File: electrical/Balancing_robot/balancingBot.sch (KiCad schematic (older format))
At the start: 21 parts, among them P101 CONN_01X04, P102 CONN_01X04, P103 CONN_01X02, SW101 SW_SPDT, U101 WRL-00691, U102 DRV8825, U103 DRV8825, U104 ArduinoProMini, U105 D24V10F5, U106 GY-521

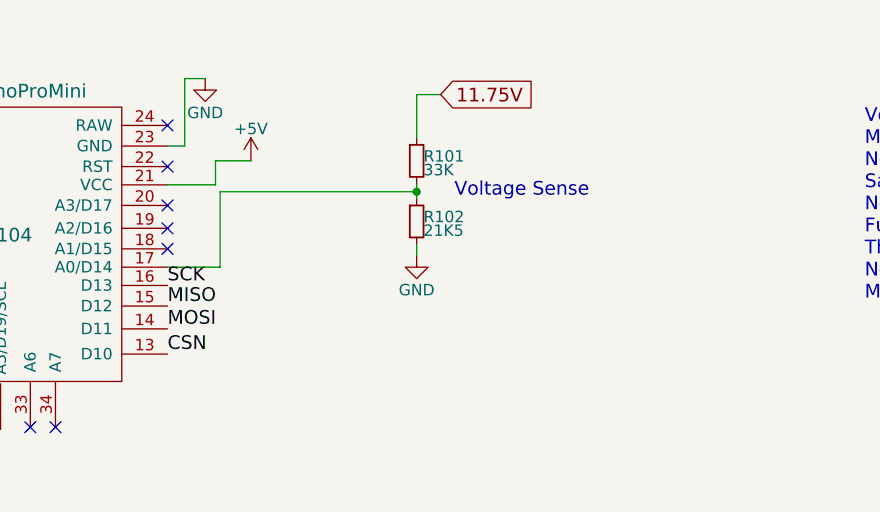
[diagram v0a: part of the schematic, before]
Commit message: finally,delayed update with a working bot
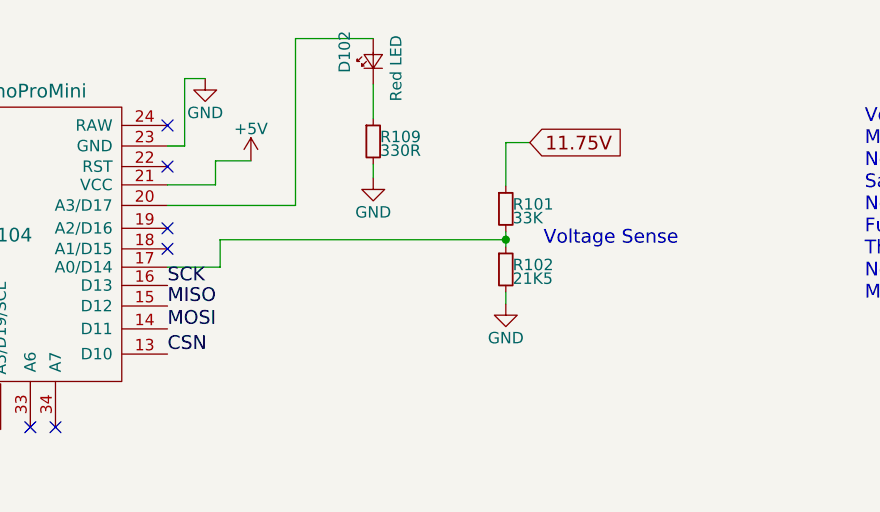
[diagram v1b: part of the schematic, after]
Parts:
- added D102: Red LED, symbol LED_Small
- added R109: 330R, symbol R_Small
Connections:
- net GND: now also R109.2
- net at U104.20 (A3/D17): now also D102.2 (A)
- new net: D102.1 (K), R109.1
- no-connect marks 26 -> 25
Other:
- moved on the sheet: R101, R102
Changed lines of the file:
@@
 NoConn ~ 4105 1855
 NoConn ~ 4105 1765
-NoConn ~ 4105 1665
-$Comp
-L GND #PWR116
+$Comp
+L GND #PWR01
 U 1 1 59559CE8
 P 9975 6160
-F 0 "#PWR116" H 9975 5910 50  0001 C CNN
+F 0 "#PWR01" H 9975 5910 50  0001 C CNN
 F 1 "GND" H 9975 6010 50  0000 C CNN
 F 2 "" H 9975 6160 50  0000 C CNN
@@
 $EndComp
 $Comp
-L +5V #PWR115
+L +5V #PWR02
 U 1 1 59559D4A
 P 9975 5700
-F 0 "#PWR115" H 9975 5550 50  0001 C CNN
+F 0 "#PWR02" H 9975 5550 50  0001 C CNN
 F 1 "+5V" H 9975 5840 50  0000 C CNN
 F 2 "" H 9975 5700 50  0000 C CNN
@@
 11.75V
 $Comp
-L GND #PWR114
+L GND #PWR03
 U 1 1 5955A15B
 P 8390 4540
-F 0 "#PWR114" H 8390 4290 50  0001 C CNN
+F 0 "#PWR03" H 8390 4290 50  0001 C CNN
 F 1 "GND" H 8390 4390 50  0000 C CNN
 F 2 "" H 8390 4540 50  0000 C CNN
@@
 $EndComp
 $Comp
-L +5V #PWR117
+L +5V #PWR04
 U 1 1 5955A1EF
 P 10055 4270
-F 0 "#PWR117" H 10055 4120 50  0001 C CNN
+F 0 "#PWR04" H 10055 4120 50  0001 C CNN
 F 1 "+5V" H 10055 4410 50  0000 C CNN
 F 2 "" H 10055 4270 50  0000 C CNN
@@
 NoConn ~ 9810 4020
 $Comp
-L +5V #PWR101
+L +5V #PWR05
 U 1 1 5955A687
 P 710 1510
-F 0 "#PWR101" H 710 1360 50  0001 C CNN
+F 0 "#PWR05" H 710 1360 50  0001 C CNN
 F 1 "+5V" H 710 1650 50  0000 C CNN
 F 2 "" H 710 1510 50  0000 C CNN
@@
 $EndComp
 $Comp
-L GND #PWR102
+L GND #PWR06
 U 1 1 5955A6E0
 P 720 1790
-F 0 "#PWR102" H 720 1540 50  0001 C CNN
+F 0 "#PWR06" H 720 1540 50  0001 C CNN
 F 1 "GND" H 720 1640 50  0000 C CNN
 F 2 "" H 720 1790 50  0000 C CNN
@@
 5V 1A
 $Comp
-L +5V #PWR105
+L +5V #PWR07
 U 1 1 5955B40F
 P 2175 1425
-F 0 "#PWR105" H 2175 1275 50  0001 C CNN
+F 0 "#PWR07" H 2175 1275 50  0001 C CNN
 F 1 "+5V" H 2175 1565 50  0000 C CNN
 F 2 "" H 2175 1425 50  0000 C CNN
@@
 11.75V
 $Comp
-L GND #PWR110
+L GND #PWR08
 U 1 1 5955B554
 P 3770 4430
-F 0 "#PWR110" H 3770 4180 50  0001 C CNN
+F 0 "#PWR08" H 3770 4180 50  0001 C CNN
 F 1 "GND" H 3770 4280 50  0000 C CNN
 F 2 "" H 3770 4430 50  0000 C CNN
@@
 $EndComp
 $Comp
-L GND #PWR108
+L GND #PWR09
 U 1 1 5955B696
 P 3160 5210
-F 0 "#PWR108" H 3160 4960 50  0001 C CNN
+F 0 "#PWR09" H 3160 4960 50  0001 C CNN
 F 1 "GND" H 3160 5060 50  0000 C CNN
 F 2 "" H 3160 5210 50  0000 C CNN
@@
 11.75V
 $Comp
-L GND #PWR109
+L GND #PWR010
 U 1 1 5955B883
 P 3735 6575
-F 0 "#PWR109" H 3735 6325 50  0001 C CNN
+F 0 "#PWR010" H 3735 6325 50  0001 C CNN
 F 1 "GND" H 3735 6425 50  0000 C CNN
 F 2 "" H 3735 6575 50  0000 C CNN
@@
 $EndComp
 $Comp
-L GND #PWR107
+L GND #PWR011
 U 1 1 5955BA2D
 P 3125 7355
-F 0 "#PWR107" H 3125 7105 50  0001 C CNN
+F 0 "#PWR011" H 3125 7105 50  0001 C CNN
 F 1 "GND" H 3125 7205 50  0000 C CNN
 F 2 "" H 3125 7355 50  0000 C CNN
@@
 M0/M1/M2:\n0 0 0 - Full Step\n1 0 0 - 1/2 Step\n0 1 0 - 1/4 Step\n1 1 0 - 1/8 Step\n0 0 1 - 1/16 Step\nInternal pull down\n
 $Comp
-L +5V #PWR104
+L +5V #PWR012
 U 1 1 59569A5C
 P 1485 4345
-F 0 "#PWR104" H 1485 4195 50  0001 C CNN
+F 0 "#PWR012" H 1485 4195 50  0001 C CNN
 F 1 "+5V" H 1485 4485 50  0000 C CNN
 F 2 "" H 1485 4345 50  0000 C CNN
@@
 L R_Small R101
 U 1 1 595697E0
-P 5195 1470
-F 0 "R101" H 5225 1490 50  0000 L CNN
-F 1 "33K" H 5225 1430 50  0000 L CNN
-F 2 "Resistors_SMD:R_0805_HandSoldering" H 5195 1470 50  0001 C CNN
-F 3 "" H 5195 1470 50  0000 C CNN
-F 4 "Value" H 5195 1470 60  0001 C CNN "Fieldname"
-	1    5195 1470
+P 5585 1680
+F 0 "R101" H 5615 1700 50  0000 L CNN
+F 1 "33K" H 5615 1640 50  0000 L CNN
+F 2 "Resistors_SMD:R_0805_HandSoldering" H 5585 1680 50  0001 C CNN
+F 3 "" H 5585 1680 50  0000 C CNN
+F 4 "Value" H 5585 1680 60  0001 C CNN "Fieldname"
+	1    5585 1680
 	1    0    0    -1
 $EndComp
@@
 L R_Small R102
 U 1 1 5956988A
-P 5195 1735
-F 0 "R102" H 5225 1755 50  0000 L CNN
-F 1 "21K5" H 5225 1695 50  0000 L CNN
-F 2 "Resistors_SMD:R_0805_HandSoldering" H 5195 1735 50  0001 C CNN
-F 3 "" H 5195 1735 50  0000 C CNN
-F 4 "Value" H 5195 1735 60  0001 C CNN "Fieldname"
-	1    5195 1735
-	1    0    0    -1
-$EndComp
-$Comp
-L GND #PWR113
+P 5585 1945
+F 0 "R102" H 5615 1965 50  0000 L CNN
+F 1 "21K5" H 5615 1905 50  0000 L CNN
+F 2 "Resistors_SMD:R_0805_HandSoldering" H 5585 1945 50  0001 C CNN
+F 3 "" H 5585 1945 50  0000 C CNN
+F 4 "Value" H 5585 1945 60  0001 C CNN "Fieldname"
+	1    5585 1945
+	1    0    0    -1
+$EndComp
+$Comp
+L GND #PWR013
 U 1 1 59569A75
-P 5195 1885
-F 0 "#PWR113" H 5195 1635 50  0001 C CNN
-F 1 "GND" H 5195 1735 50  0000 C CNN
-F 2 "" H 5195 1885 50  0000 C CNN
-F 3 "" H 5195 1885 50  0000 C CNN
-	1    5195 1885
-	1    0    0    -1
-$EndComp
-Text GLabel 5300 1180 2    60   Input ~ 0
+P 5585 2095
+F 0 "#PWR013" H 5585 1845 50  0001 C CNN
+F 1 "GND" H 5585 1945 50  0000 C CNN
+F 2 "" H 5585 2095 50  0000 C CNN
+F 3 "" H 5585 2095 50  0000 C CNN
+	1    5585 2095
+	1    0    0    -1
+$EndComp
+Text GLabel 5690 1390 2    60   Input ~ 0
 11.75V
-Text Notes 5360 1635 0    60   ~ 0
+Text Notes 5750 1845 0    60   ~ 0
 Voltage Sense
 Text Label 2795 1695 2    60   ~ 0
@@
 NoConn ~ 3125 7180
 $Comp
-L GND #PWR111
+L GND #PWR014
 U 1 1 59AC80BA
 P 4270 1110
-F 0 "#PWR111" H 4270 860 50  0001 C CNN
+F 0 "#PWR014" H 4270 860 50  0001 C CNN
 F 1 "GND" H 4270 960 50  0000 C CNN
 F 2 "" H 4270 1110 50  0000 C CNN
@@
 $EndComp
 $Comp
-L +5V #PWR112
+L +5V #PWR015
 U 1 1 59AC8320
 P 4470 1470
-F 0 "#PWR112" H 4470 1320 50  0001 C CNN
+F 0 "#PWR015" H 4470 1320 50  0001 C CNN
 F 1 "+5V" H 4470 1610 50  0000 C CNN
 F 2 "" H 4470 1470 50  0000 C CNN
@@
 $EndComp
 $Comp
-L GND #PWR106
+L GND #PWR016
 U 1 1 59AC848A
 P 2370 1665
-F 0 "#PWR106" H 2370 1415 50  0001 C CNN
+F 0 "#PWR016" H 2370 1415 50  0001 C CNN
 F 1 "GND" H 2370 1515 50  0000 C CNN
 F 2 "" H 2370 1665 50  0000 C CNN
@@
 Connection ~ 8390 4240
 Wire Wire Line
-	5300 1180 5195 1180
-Wire Wire Line
-	5195 1180 5195 1370
-Wire Wire Line
-	5195 1570 5195 1635
-Wire Wire Line
-	5195 1835 5195 1885
+	5690 1390 5585 1390
+Wire Wire Line
+	5585 1390 5585 1580
+Wire Wire Line
+	5585 1780 5585 1845
+Wire Wire Line
+	5585 2045 5585 2095
 Wire Wire Line
 	4105 1935 4335 1935
 Wire Wire Line
-	4335 1935 4335 1605
-Wire Wire Line
-	4335 1605 5195 1605
-Connection ~ 5195 1605
+	4335 1815 5585 1815
+Connection ~ 5585 1815
 Wire Wire Line
 	3120 6200 3120 6210
@@
 Connection ~ 1825 4360
 $Comp
-L +5V #PWR103
+L +5V #PWR017
 U 1 1 59ADD131
 P 1450 6490
-F 0 "#PWR103" H 1450 6340 50  0001 C CNN
+F 0 "#PWR017" H 1450 6340 50  0001 C CNN
 F 1 "+5V" H 1450 6630 50  0000 C CNN
 F 2 "" H 1450 6490 50  0000 C CNN
@@
 Text Notes 4370 7170 0    60   ~ 0
 Green\nBlack\nRed\nBlue
+Wire Wire Line
+	4335 1935 4335 1815
+$Comp
+L R_Small R109
+U 1 1 5A80AAAD
+P 5005 1385
+F 0 "R109" H 5035 1405 50  0000 L CNN
+F 1 "330R" H 5035 1345 50  0000 L CNN
+F 2 "" H 5005 1385 50  0000 C CNN
+F 3 "" H 5005 1385 50  0000 C CNN
+F 4 "Value" H 5005 1385 60  0001 C CNN "Fieldname"
+	1    5005 1385
+	1    0    0    -1
+$EndComp
+$Comp
+L LED_Small D102
+U 1 1 5A80AB29
+P 5005 1035
+F 0 "D102" H 4955 1160 50  0000 L CNN
+F 1 "Red LED" H 4830 935 50  0000 L CNN
+F 2 "" V 5005 1035 50  0000 C CNN
+F 3 "" V 5005 1035 50  0000 C CNN
+F 4 "Value" H 5005 1035 60  0001 C CNN "Fieldname"
+	1    5005 1035
+	0    -1   -1   0
+$EndComp
+$Comp
+L GND #PWR018
+U 1 1 5A80ACDE
+P 5005 1545
+F 0 "#PWR018" H 5005 1295 50  0001 C CNN
+F 1 "GND" H 5005 1395 50  0000 C CNN
+F 2 "" H 5005 1545 50  0000 C CNN
+F 3 "" H 5005 1545 50  0000 C CNN
+	1    5005 1545
+	1    0    0    -1
+$EndComp
+Wire Wire Line
+	5005 1485 5005 1545
+Wire Wire Line
+	5005 1135 5005 1285
+Wire Wire Line
+	4105 1665 4665 1665
+Wire Wire Line
+	4665 1665 4665 935
+Wire Wire Line
+	4665 935  5005 935
 $EndSCHEMATC
